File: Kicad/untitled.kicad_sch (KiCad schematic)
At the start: 24 parts, among them J1 Thermistor, U1 STM32G431C8Tx, U2 AS5047P, Y1 24MHz

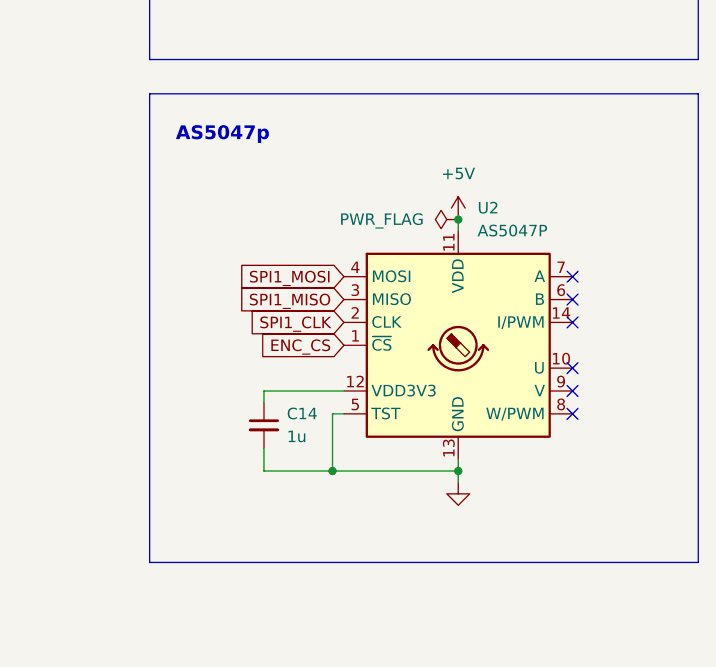
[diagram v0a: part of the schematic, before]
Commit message: commit
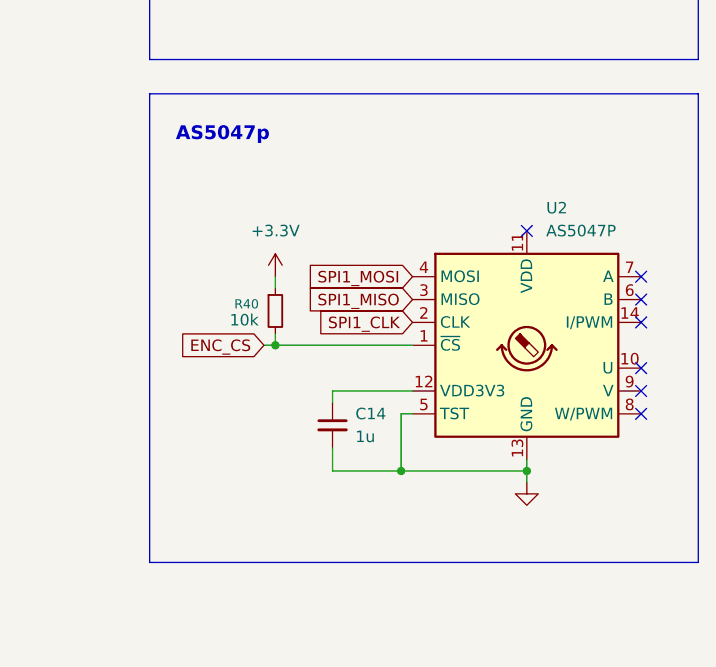
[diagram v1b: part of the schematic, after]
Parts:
- added R40: 10k, Resistor_SMD:R_0402_1005Metric, symbol Device:R_Small
- R3, R4: footprint Resistor_SMD:R_01005_0402Metric -> Resistor_SMD:R_0402_1005Metric
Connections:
- net +3.3V: now also R40.1
- net ENC_CS: now also R40.2
- net +5V: no longer names the net of U2.11 (VDD)
- no-connect marks 12 -> 13
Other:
- moved on the sheet: C14, U2
